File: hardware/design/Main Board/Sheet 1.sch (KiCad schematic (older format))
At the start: 2 parts

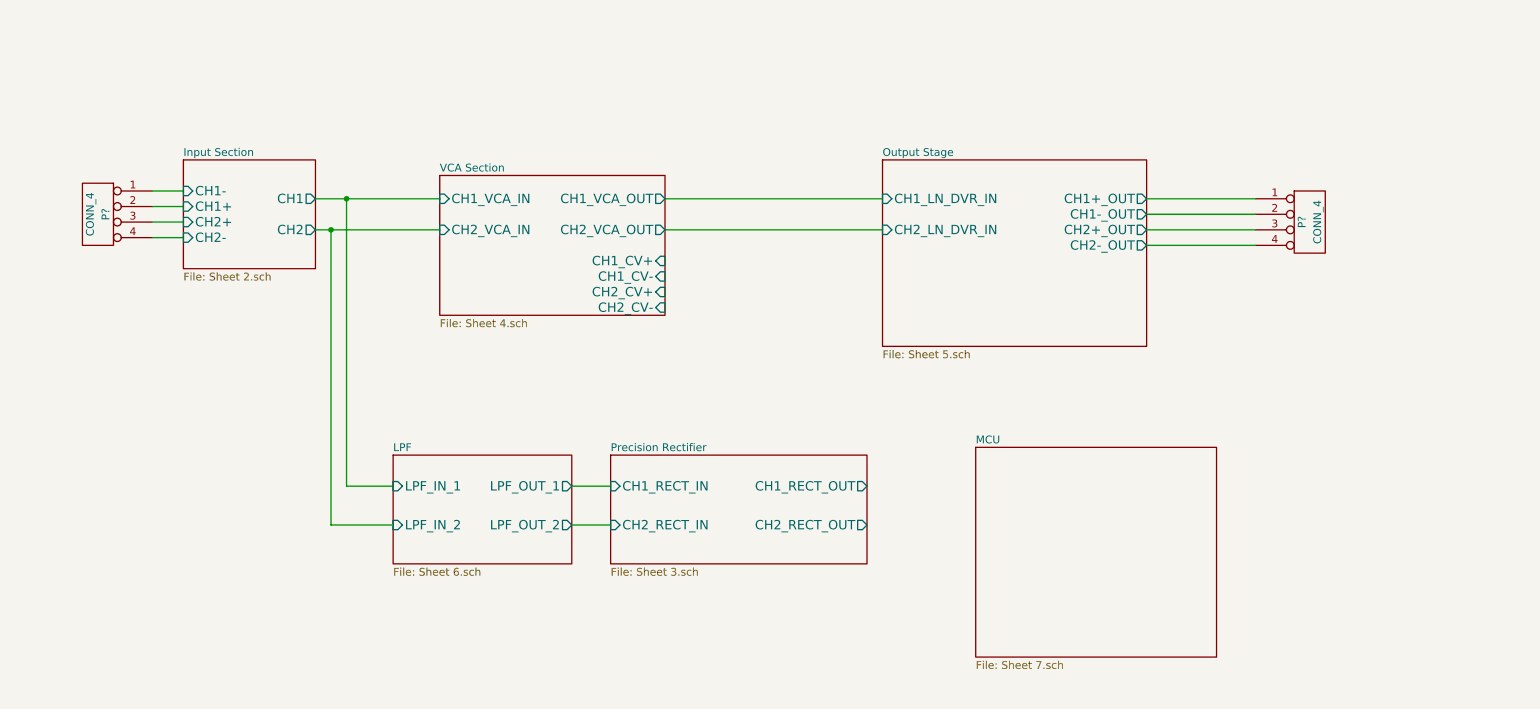
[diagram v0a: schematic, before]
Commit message: Version 1.0
Wrapped up design. Version for Detailed Design Review.
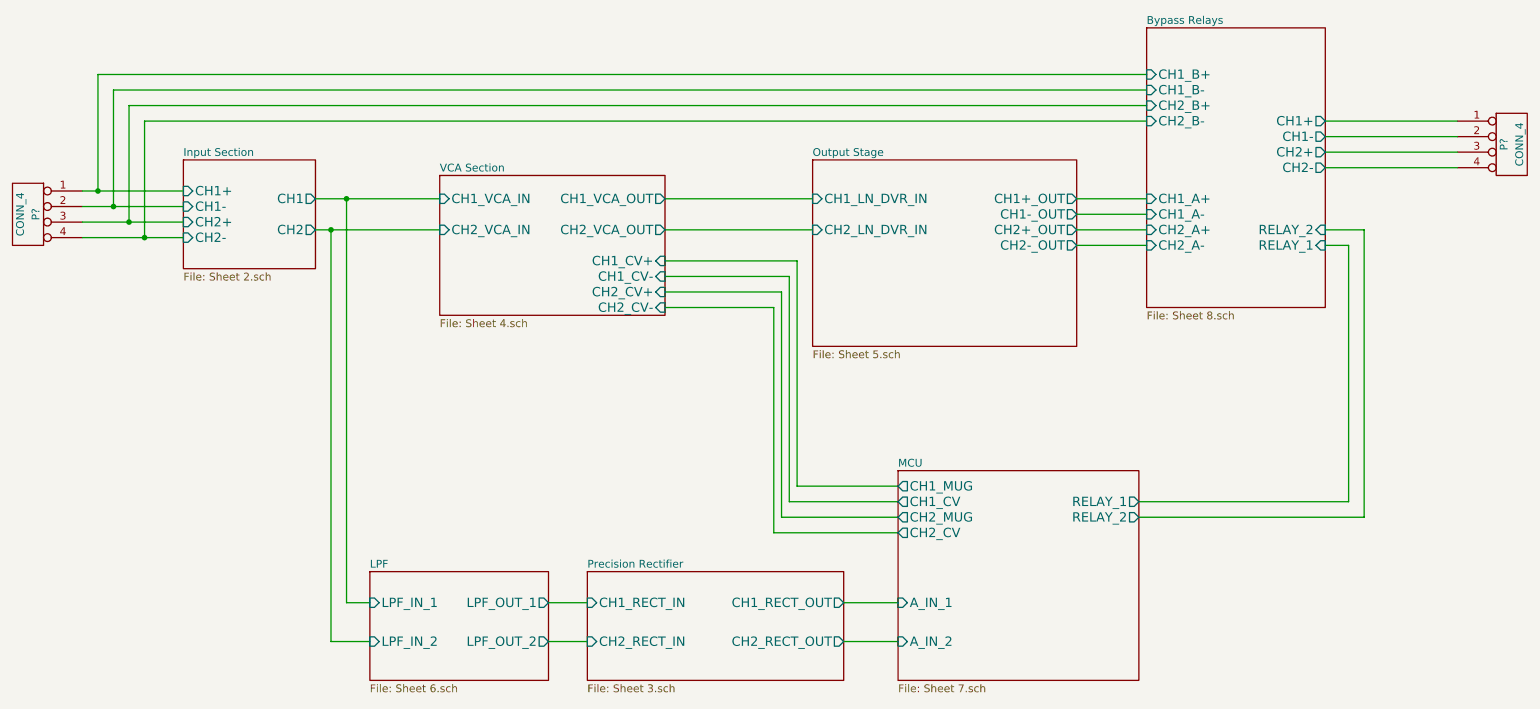
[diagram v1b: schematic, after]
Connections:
- net Input Section/CH1+ renamed Bypass Relays/CH1_B-
- net Input Section/CH1- renamed Bypass Relays/CH1_B+
- net Input Section/CH2+ renamed Bypass Relays/CH2_B+
- net Input Section/CH2- renamed Bypass Relays/CH2_B-
- net Output Stage/CH1+_OUT renamed Bypass Relays/CH1+
- net Output Stage/CH1-_OUT renamed Bypass Relays/CH1-
- net Output Stage/CH2+_OUT renamed Bypass Relays/CH2+
- net Output Stage/CH2-_OUT renamed Bypass Relays/CH2-
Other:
- moved on the sheet: P?
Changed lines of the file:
@@
 EELAYER 27 0
 EELAYER END
-$Descr A4 11693 8268
+$Descr USLetter 11000 8500
 encoding utf-8
-Sheet 1 8
-Title ""
-Date "6 may 2014"
-Rev ""
-Comp ""
-Comment1 ""
+Sheet 1 9
+Title "Hybrid Audio Dynamics Processor"
+Date "10 may 2014"
+Rev "1.0"
+Comp "P14345"
+Comment1 "Top Level Schematic"
 Comment2 ""
 Comment3 ""
@@
 L CONN_4 P?
 U 1 1 534DB1BE
-P 1150 2600
-F 0 "P?" V 1100 2600 50  0000 C CNN
-F 1 "CONN_4" V 1200 2600 50  0000 C CNN
-F 2 "" H 1150 2600 60  0000 C CNN
-F 3 "" H 1150 2600 60  0000 C CNN
-	1    1150 2600
+P 700 2600
+F 0 "P?" V 650 2600 50  0000 C CNN
+F 1 "CONN_4" V 750 2600 50  0000 C CNN
+F 2 "" H 700 2600 60  0000 C CNN
+F 3 "" H 700 2600 60  0000 C CNN
+	1    700  2600
 	-1   0    0    -1
 $EndComp
@@
 F0 "Input Section" 50
 F1 "Sheet 2.sch" 50
-F2 "CH1-" I L 1700 2450 60
-F3 "CH1+" I L 1700 2550 60
+F2 "CH1-" I L 1700 2550 60
+F3 "CH1+" I L 1700 2450 60
 F4 "CH2+" I L 1700 2650 60
 F5 "CH2-" I L 1700 2750 60
@@
 $EndSheet
 Wire Wire Line
-	1500 2450 1700 2450
-Wire Wire Line
-	1500 2550 1700 2550
-Wire Wire Line
-	1500 2650 1700 2650
-Wire Wire Line
-	1500 2750 1700 2750
-$Sheet
-S 4450 4150 1650 700
+	1050 2650 1700 2650
+Wire Wire Line
+	1050 2750 1700 2750
+$Sheet
+S 4300 4900 1650 700
 U 534DCE54
 F0 "Precision Rectifier" 50
 F1 "Sheet 3.sch" 50
-F2 "CH1_RECT_IN" I L 4450 4350 60
-F3 "CH2_RECT_IN" I L 4450 4600 60
-F4 "CH1_RECT_OUT" O R 6100 4350 60
-F5 "CH2_RECT_OUT" O R 6100 4600 60
+F2 "CH1_RECT_IN" I L 4300 5100 60
+F3 "CH2_RECT_IN" I L 4300 5350 60
+F4 "CH1_RECT_OUT" O R 5950 5100 60
+F5 "CH2_RECT_OUT" O R 5950 5350 60
 $EndSheet
 Wire Wire Line
@@
 $EndSheet
 $Sheet
-S 6200 2250 1700 1200
+S 5750 2250 1700 1200
 U 534F2525
 F0 "Output Stage" 50
 F1 "Sheet 5.sch" 50
-F2 "CH1_LN_DVR_IN" I L 6200 2500 60
-F3 "CH1+_OUT" O R 7900 2500 60
-F4 "CH1-_OUT" O R 7900 2600 60
-F5 "CH2_LN_DVR_IN" I L 6200 2700 60
-F6 "CH2+_OUT" O R 7900 2700 60
-F7 "CH2-_OUT" O R 7900 2800 60
-$EndSheet
-Wire Wire Line
-	4800 2500 6200 2500
-Wire Wire Line
-	4800 2700 6200 2700
+F2 "CH1_LN_DVR_IN" I L 5750 2500 60
+F3 "CH1+_OUT" O R 7450 2500 60
+F4 "CH1-_OUT" O R 7450 2600 60
+F5 "CH2_LN_DVR_IN" I L 5750 2700 60
+F6 "CH2+_OUT" O R 7450 2700 60
+F7 "CH2-_OUT" O R 7450 2800 60
+$EndSheet
 $Comp
 L CONN_4 P?
 U 1 1 5362E417
-P 8950 2650
-F 0 "P?" V 8900 2650 50  0000 C CNN
-F 1 "CONN_4" V 9000 2650 50  0000 C CNN
-F 2 "" H 8950 2650 60  0000 C CNN
-F 3 "" H 8950 2650 60  0000 C CNN
-	1    8950 2650
+P 10250 2150
+F 0 "P?" V 10200 2150 50  0000 C CNN
+F 1 "CONN_4" V 10300 2150 50  0000 C CNN
+F 2 "" H 10250 2150 60  0000 C CNN
+F 3 "" H 10250 2150 60  0000 C CNN
+	1    10250 2150
 	1    0    0    -1
 $EndComp
 $Sheet
-S 3050 4150 1150 700
+S 2900 4900 1150 700
 U 5362F285
 F0 "LPF" 50
 F1 "Sheet 6.sch" 50
-F2 "LPF_IN_1" I L 3050 4350 60
-F3 "LPF_IN_2" I L 3050 4600 60
-F4 "LPF_OUT_1" O R 4200 4350 60
-F5 "LPF_OUT_2" O R 4200 4600 60
-$EndSheet
-Wire Wire Line
-	3050 4350 2750 4350
-Wire Wire Line
-	2750 4350 2750 2500
+F2 "LPF_IN_1" I L 2900 5100 60
+F3 "LPF_IN_2" I L 2900 5350 60
+F4 "LPF_OUT_1" O R 4050 5100 60
+F5 "LPF_OUT_2" O R 4050 5350 60
+$EndSheet
+Wire Wire Line
+	2750 2500 2750 5100
 Connection ~ 2750 2500
 Wire Wire Line
-	2650 2700 2650 4600
-Wire Wire Line
-	2650 4600 3050 4600
+	2650 2700 2650 5350
 Connection ~ 2650 2700
 Wire Wire Line
-	4200 4350 4450 4350
-Wire Wire Line
-	4200 4600 4450 4600
-Wire Wire Line
-	8600 2500 7900 2500
-Wire Wire Line
-	8600 2600 7900 2600
-Wire Wire Line
-	8600 2700 7900 2700
-Wire Wire Line
-	8600 2800 7900 2800
-$Sheet
-S 6800 4100 1550 1350
+	4050 5100 4300 5100
+Wire Wire Line
+	4050 5350 4300 5350
+$Sheet
+S 6300 4250 1550 1350
 U 53665ABB
 F0 "MCU" 50
 F1 "Sheet 7.sch" 50
-$EndSheet
+F2 "A_IN_1" I L 6300 5100 60
+F3 "A_IN_2" I L 6300 5350 60
+F4 "RELAY_1" O R 7850 4450 60
+F5 "RELAY_2" O R 7850 4550 60
+F6 "CH1_CV" O L 6300 4450 60
+F7 "CH2_CV" O L 6300 4650 60
+F8 "CH1_MUG" O L 6300 4350 60
+F9 "CH2_MUG" O L 6300 4550 60
+$EndSheet
+Wire Wire Line
+	2750 5100 2900 5100
+Wire Wire Line
+	2650 5350 2900 5350
+Wire Wire Line
+	5950 5100 6300 5100
+Wire Wire Line
+	5950 5350 6300 5350
+Wire Wire Line
+	6300 4350 5650 4350
+Wire Wire Line
+	5650 4350 5650 2900
+Wire Wire Line
+	5650 2900 4800 2900
+Wire Wire Line
+	6300 4450 5600 4450
+Wire Wire Line
+	5600 4450 5600 3000
+Wire Wire Line
+	5600 3000 4800 3000
+Wire Wire Line
+	6300 4550 5550 4550
+Wire Wire Line
+	5550 4550 5550 3100
+Wire Wire Line
+	5550 3100 4800 3100
+Wire Wire Line
+	6300 4650 5500 4650
+Wire Wire Line
+	5500 4650 5500 3200
+Wire Wire Line
+	5500 3200 4800 3200
+$Sheet
+S 7900 1400 1150 1800
+U 536F9075
+F0 "Bypass Relays" 50
+F1 "Sheet 8.sch" 50
+F2 "RELAY_1" I R 9050 2800 60
+F3 "RELAY_2" I R 9050 2700 60
+F4 "CH1_A+" I L 7900 2500 60
+F5 "CH1_B+" I L 7900 1700 60
+F6 "CH1_A-" I L 7900 2600 60
+F7 "CH1_B-" I L 7900 1800 60
+F8 "CH1+" O R 9050 2000 60
+F9 "CH1-" O R 9050 2100 60
+F10 "CH2_A+" I L 7900 2700 60
+F11 "CH2_B+" I L 7900 1900 60
+F12 "CH2_A-" I L 7900 2800 60
+F13 "CH2_B-" I L 7900 2000 60
+F14 "CH2+" O R 9050 2200 60
+F15 "CH2-" O R 9050 2300 60
+$EndSheet
+Wire Wire Line
+	1050 2450 1700 2450
+Wire Wire Line
+	1050 2550 1700 2550
+Wire Wire Line
+	7900 1700 1150 1700
+Wire Wire Line
+	1150 1700 1150 2450
+Connection ~ 1150 2450
+Wire Wire Line
+	7900 1800 1250 1800
+Wire Wire Line
+	1250 1800 1250 2550
+Connection ~ 1250 2550
+Wire Wire Line
+	7900 1900 1350 1900
+Wire Wire Line
+	1350 1900 1350 2650
+Connection ~ 1350 2650
+Wire Wire Line
+	7900 2000 1450 2000
+Wire Wire Line
+	1450 2000 1450 2750
+Connection ~ 1450 2750
+Wire Wire Line
+	7450 2800 7900 2800
+Wire Wire Line
+	7450 2700 7900 2700
+Wire Wire Line
+	7450 2600 7900 2600
+Wire Wire Line
+	7450 2500 7900 2500
+Wire Wire Line
+	7850 4450 9200 4450
+Wire Wire Line
+	9200 4450 9200 2800
+Wire Wire Line
+	9200 2800 9050 2800
+Wire Wire Line
+	9050 2700 9300 2700
+Wire Wire Line
+	9300 2700 9300 4550
+Wire Wire Line
+	9300 4550 7850 4550
+Wire Wire Line
+	9050 2000 9900 2000
+Wire Wire Line
+	9050 2100 9900 2100
+Wire Wire Line
+	9050 2200 9900 2200
+Wire Wire Line
+	9050 2300 9900 2300
+Wire Wire Line
+	4800 2500 5750 2500
+Wire Wire Line
+	4800 2700 5750 2700
 $EndSCHEMATC
